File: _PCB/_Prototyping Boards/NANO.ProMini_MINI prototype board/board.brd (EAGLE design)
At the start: 58.2 x 41 mm, 19 parts, among them T1_5MM 5mm

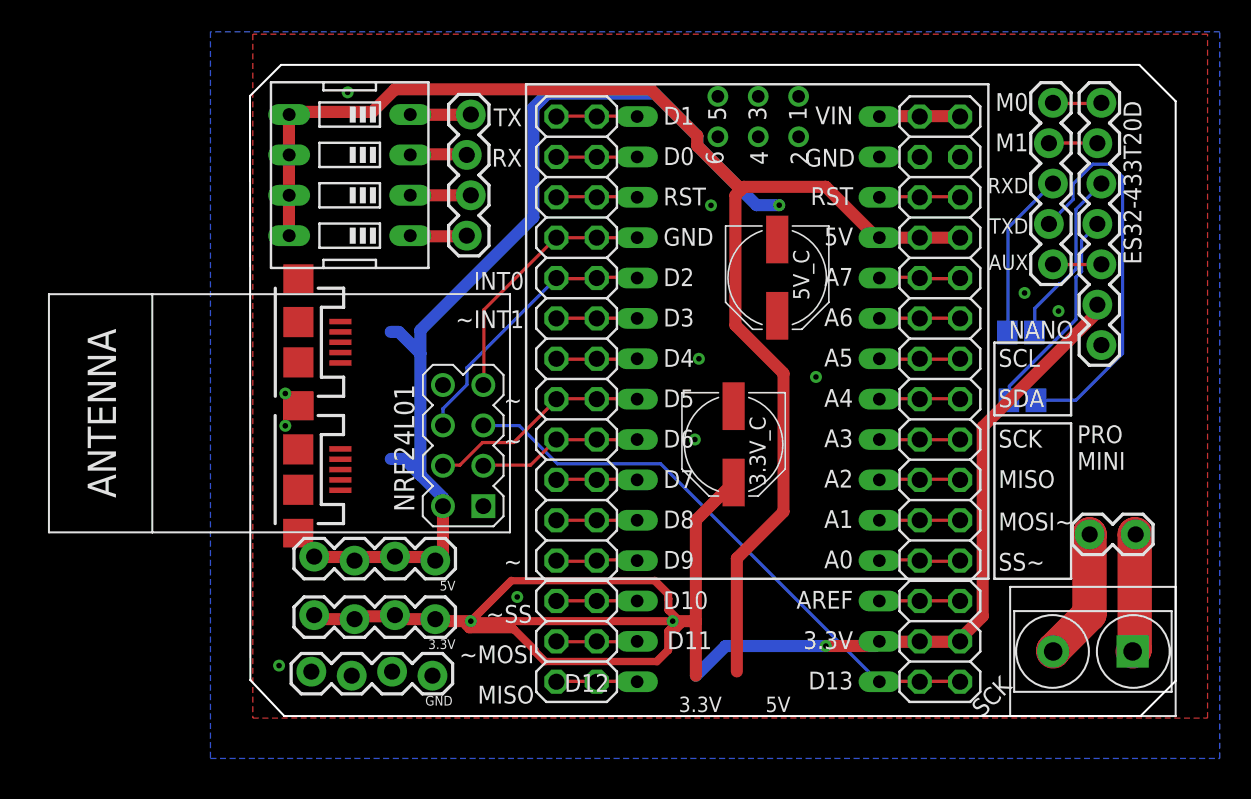
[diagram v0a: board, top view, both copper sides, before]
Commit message: proto board update
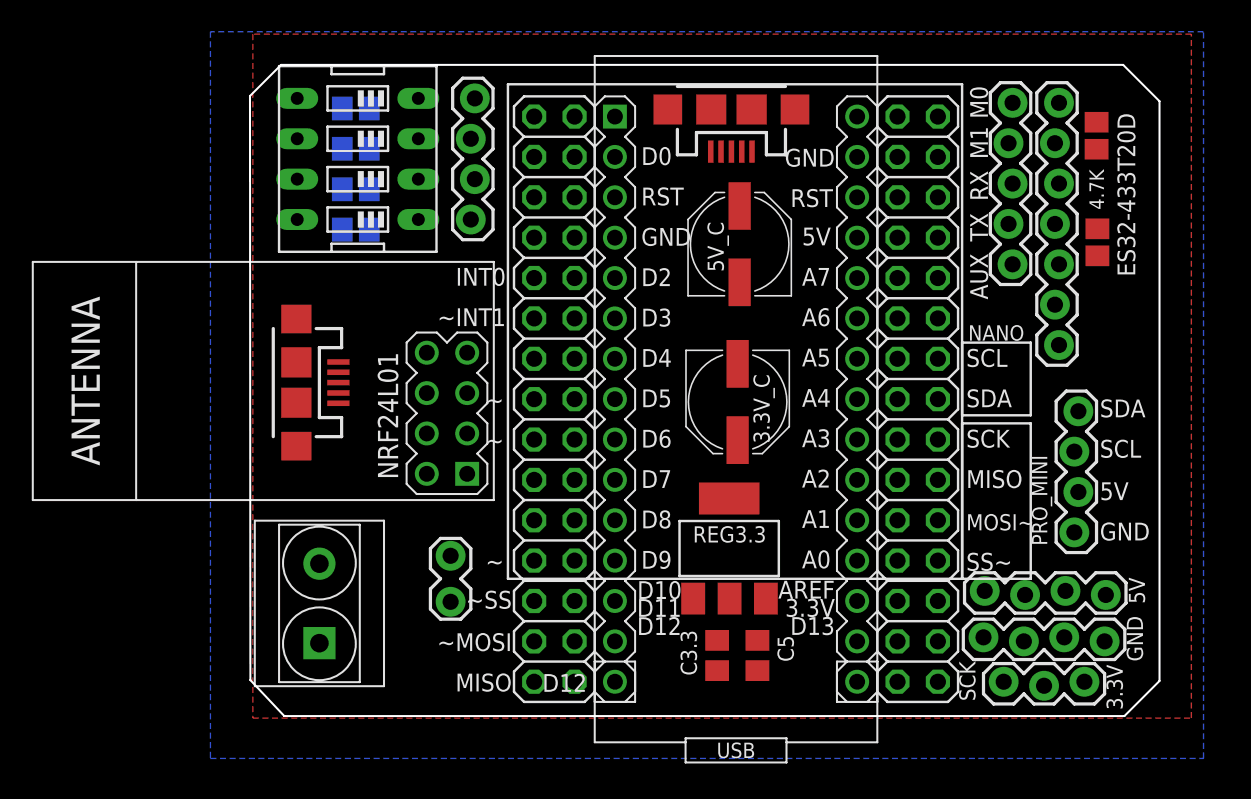
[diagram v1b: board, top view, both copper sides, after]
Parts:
- added C3.3, C5: (no value), rcl:C0805
- added I2C_1: (no value), SparkFun-Connectors:1X04_LOCK
- added R3, R4, R5, R6: 10k, rcl:R2012
- added REG3.3: REG1117, burr-brown:SOT223
- 3.3V: device SparkFun-Connectors:1X04_LOCK -> SparkFun-Connectors:1X03_LOCK
- NANO: value NANO -> ARDUINO-NANO-3.0; device Arduino-clone:NANO -> diy-modules:ARDUINO-NANO-3.0
- moved T1_5MM 48.8 mm to (4.32, 7.21), turned to 180 degrees
- moved PIN1 40.4 mm to (12.6, 10.0), turned to 270 degrees
- moved 3.3V 36.0 mm to (47.4, 2.16), turned to 0 degrees
- moved MICRO_2 35.4 mm to (30.2, 38.3), turned to 90 degrees
- moved GND 34.7 mm to (46.1, 4.95), turned to 0 degrees
- moved 5V 34.6 mm to (46.2, 7.87), turned to 0 degrees
- moved R2 13.3 mm to (53.2, 36.6), flipped to the top, turned to 270 degrees
- moved R1 11.0 mm to (53.3, 29.9), flipped to the top, turned to 90 degrees
- moved NANO 8.96 mm to (30.5, 20.1), turned to 90 degrees
- moved 5V_C 3.17 mm to (30.8, 29.8), turned to 90 degrees
- moved 3.3V_C 2.68 mm to (30.6, 19.9)
- moved ES32-433T20D 2.67 mm to (50.7, 38.7)
- moved MICRO_1 2.54 mm to (2.87, 21.1)
- moved J1 2.54 mm to (47.8, 38.7)
- moved NRF24L01 2.27 mm to (0.91, 21.7)
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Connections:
- net N$1 renamed M1
- net N$12 renamed M0
- net N$15 renamed ES32_TXD
- net N$22 renamed ES32_AUX
- net N$38 renamed ES32_RXD
- removed net SDA_GY521: NANO.A4, PH1.15, PH1.16
- new net SDA: I2C_1.4, NANO.J2.8, PH1.15, PH1.16
- net 3.3V: now also C3.3.2, NANO.J2.14, REG3.3.2; no longer 3.3V.4, NANO.3.3V
- net 5V: now also C5.1, I2C_1.2, NANO.J2.4, REG3.3.3; no longer NANO.5V
- net A5: now also I2C_1.3, NANO.J2.7; no longer NANO.A5
- net A6: now also NANO.J2.6; no longer NANO.A6
- net A7: now also NANO.J2.5; no longer NANO.A7
- net CE_NRF: now also NANO.J1.9; no longer NANO.D6
- net CSN_NRF: now also NANO.J1.8; no longer NANO.D5
- net GND: now also C3.3.1, C5.2, I2C_1.1, NANO.J2.2, R3.1, R4.1, R5.1, R6.1, REG3.3.1; no longer NANO.GND, NANO.ICSP6
- net MISO_NRF: now also NANO.J1.4; no longer NANO.GND1
- net MOSI_NRF: now also NANO.J1.5; no longer NANO.D2
- net N$16: now also NANO.J1.15; no longer NANO.D12
- net N$17: now also NANO.J1.14; no longer NANO.D11
- net N$18: now also NANO.J1.13; no longer NANO.D10
- net N$19: now also NANO.J1.12; no longer NANO.D9
- net N$20: now also NANO.J1.11; no longer NANO.D8
- net N$21: now also NANO.J1.10; no longer NANO.D7
- net N$24: now also NANO.J1.7; no longer NANO.D4
- net N$25: now also NANO.J1.6; no longer NANO.D3
- net N$28: now also NANO.J1.3; no longer NANO.RST1
- net N$29: now also NANO.J1.2; no longer NANO.RX1
- net N$3: now also NANO.J2.13; no longer NANO.AREF
- net N$30: now also NANO.J1.1; no longer NANO.TX0
- net N$39: now also R3.2
- net N$4: now also NANO.J2.12; no longer NANO.A0
- net N$40: now also R4.2
- net N$41: now also R5.2
- net N$42: now also R6.2
- net N$5: now also NANO.J2.11; no longer NANO.A1
- net N$6: now also NANO.J2.10; no longer NANO.A2
- net N$7: now also NANO.J2.9; no longer NANO.A3
- net RST: now also NANO.J2.3; no longer NANO.RST
- net SCK_NRF: now also NANO.J2.15; no longer NANO.D13
- net VIN: now also NANO.J2.1; no longer NANO.RAW
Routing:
- net 5V: track 151.3 -> 0.00 mm, vias 1 -> 0
- net 3.3V: track 112.2 -> 0.00 mm, vias 3 -> 0
- net SCK_NRF: track 36.7 -> 0.00 mm
- net N$13: track 24.9 -> 0.00 mm
- net MOSI_NRF: track 17.4 -> 0.00 mm
- net MISO_NRF: track 16.3 -> 0.00 mm
- net CSN_NRF: track 14.0 -> 0.00 mm
- net ES32_TXD: track 13.4 -> 0.00 mm
- net ES32_RXD: track 11.2 -> 0.00 mm
- net N$14: track 10.6 -> 0.00 mm
- net CE_NRF: track 10.4 -> 0.00 mm
- net N$26: track 8.32 -> 0.00 mm
- net N$23: track 7.48 -> 0.00 mm
- net N$4: track 5.20 -> 0.00 mm
- net A7: track 5.20 -> 0.00 mm
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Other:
- board size 58.2 x 41 mm -> 57.2 x 41 mm
- board text added: "PRO_MINI"
- board text removed: "1"
- board text removed: "2"
- board text removed: "3"
- board text removed: "4"
- board text removed: "5"
- board text removed: "6"
- board text removed: "D1"
- board text removed: "PRO MINI"
- board text removed: "RXD"
- board text removed: "TXD"
- board text removed: "VIN"
